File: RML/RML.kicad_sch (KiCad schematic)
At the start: 14 parts, among them Q101 PMOS, U101 LMC555xM, U102 641964-1, U103 641964-1, U104 LM555xM, U3 SFH617A-1

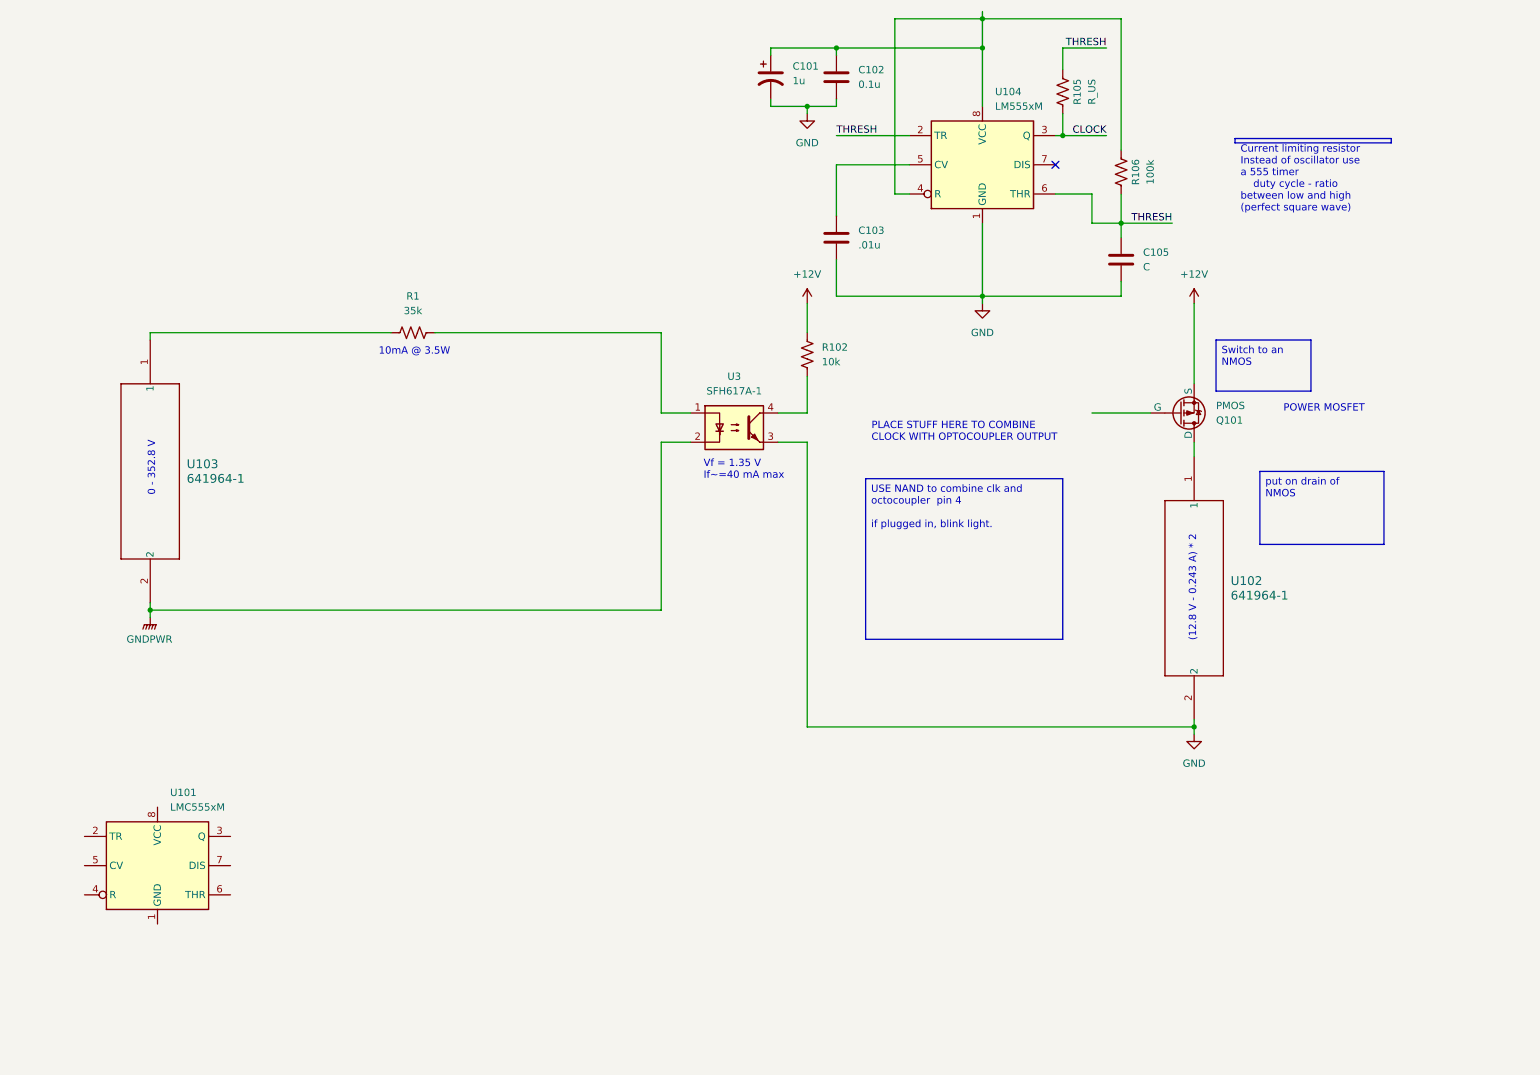
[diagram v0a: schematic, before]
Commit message: RML Notes
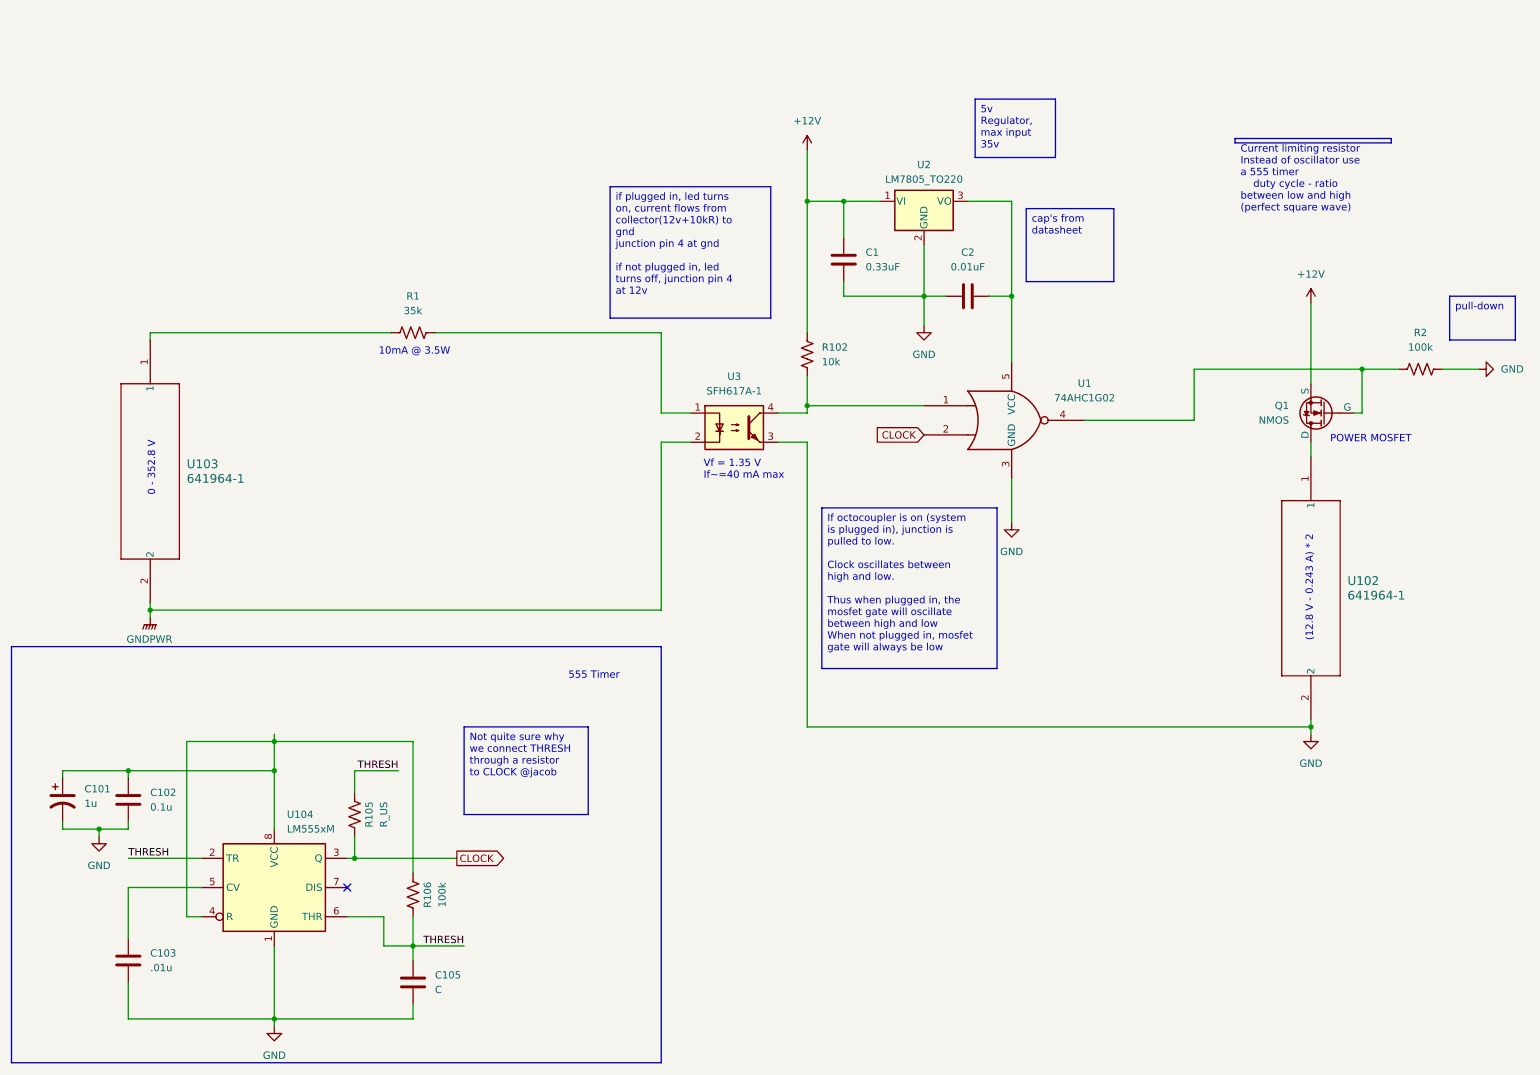
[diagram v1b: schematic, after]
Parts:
- removed Q101: PMOS, symbol Simulation_SPICE:PMOS
- removed U101: LMC555xM, Package_SO:SOIC-8_3.9x4.9mm_P1.27mm, symbol Timer:LMC555xM
- added C1: 0.33uF, symbol Device:C
- added C2: 0.01uF, symbol Device:C
- added Q1: NMOS, symbol Simulation_SPICE:NMOS
- added R2: 100k, symbol Device:R_US
- added U1: 74AHC1G02, symbol 74xGxx:74AHC1G02
- added U2: LM7805_TO220, Package_TO_SOT_THT:TO-220-3_Vertical, symbol Regulator_Linear:LM7805_TO220
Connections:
- net +12V: now also C1.1, Q1.3 (S), U2.1 (VI)
- net CLOCK: now also U1.2
- net GND: now also C1.2, C2.2, R2.2, U1.3 (GND), U2.2 (GND)
- net at U102.1: now also Q1.1 (D)
- net at R102.2, U3.4: now also U1.1
- new net: C2.1, U1.5 (VCC), U2.3 (VO)
- new net: Q1.2 (G), R2.1, U1.4
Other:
- note added: "555 Timer"
- note removed: "PLACE STUFF HERE TO COMBINE CLOCK WITH OPTOCOUPLER OUTPUT"
- moved on the sheet: C101, C102, C103, C105, R105, R106, U102, U104
